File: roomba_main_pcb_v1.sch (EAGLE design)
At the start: 14 parts, among them J1 J25MM

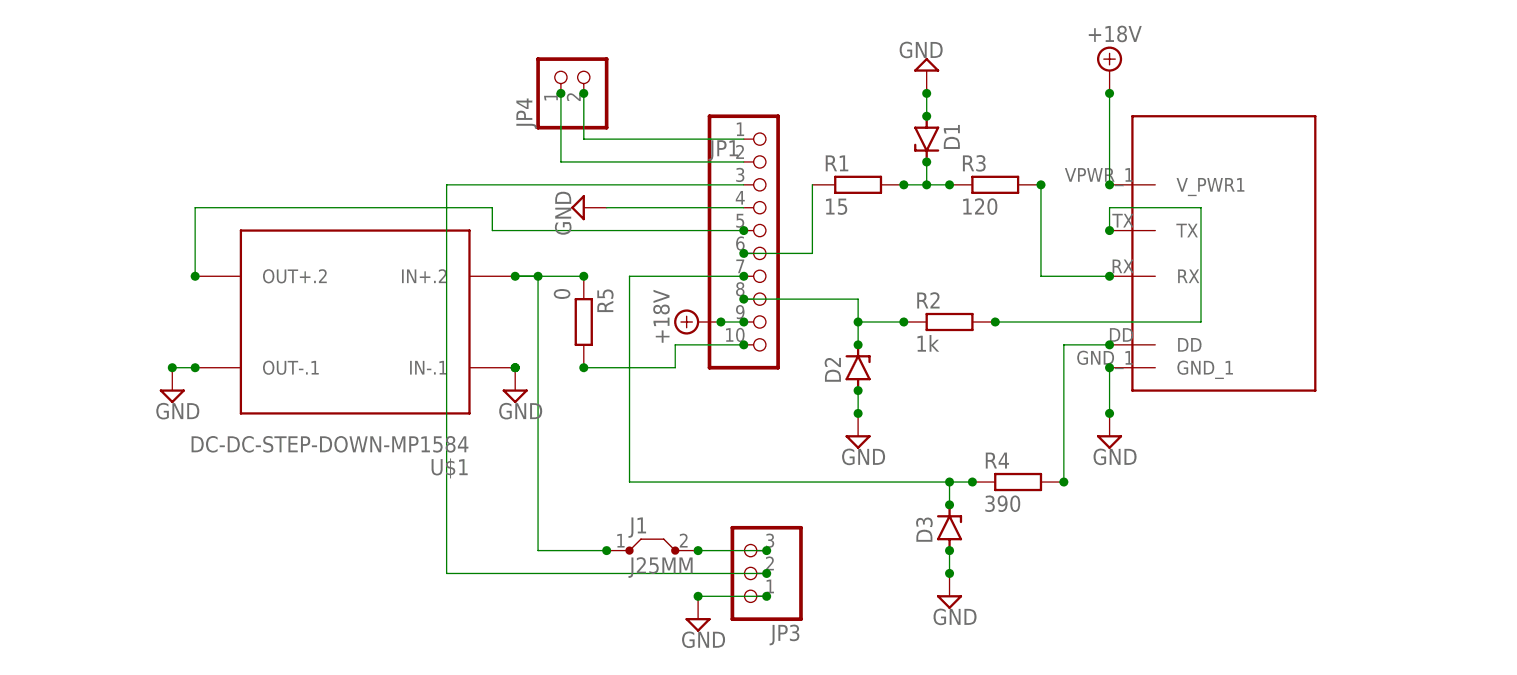
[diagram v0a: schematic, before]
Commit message: 1.1
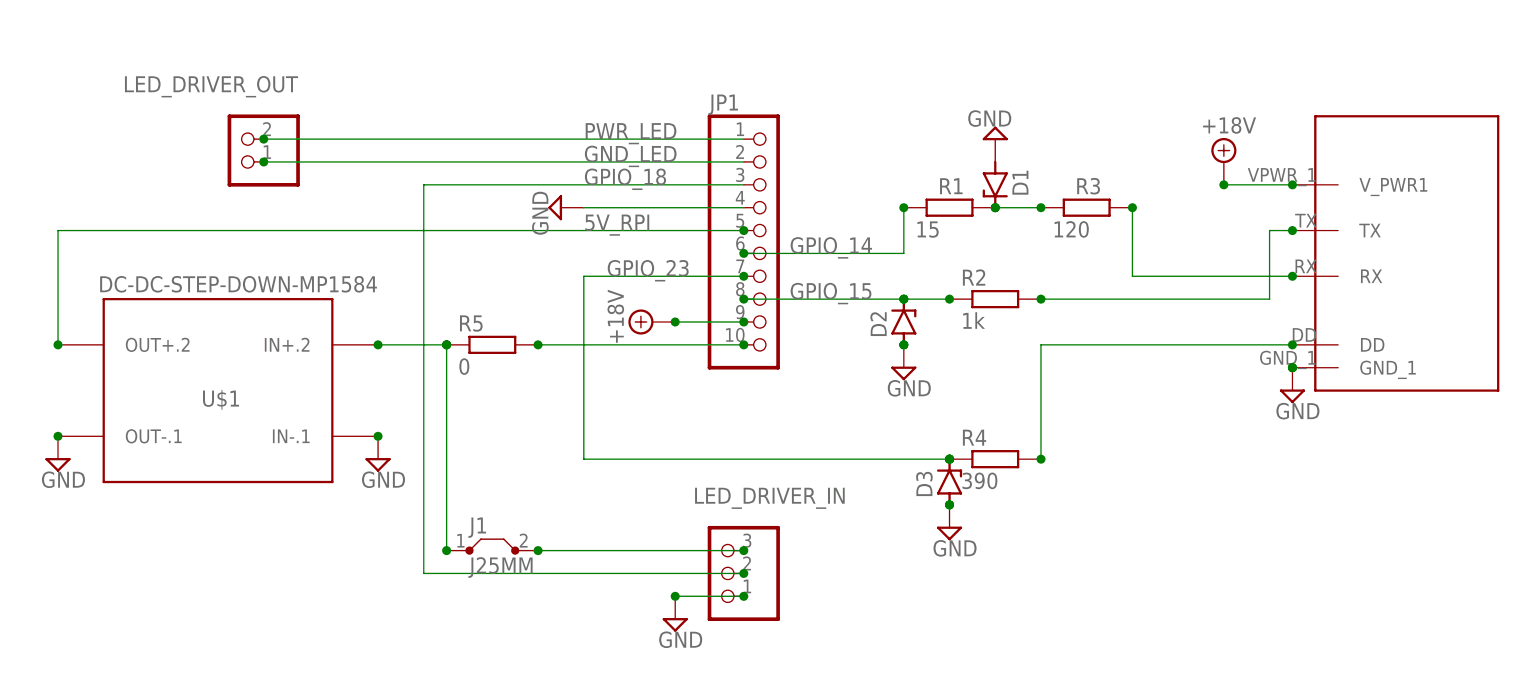
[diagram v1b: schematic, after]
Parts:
- removed JP3: (no value), pinhead:PINHD-1X3
- removed JP4: (no value), pinhead:PINHD-1X2
- removed U$3: 7_PIN, M_wifi:7_PIN
- added LED_DRIVER_IN: (no value), pinhead:PINHD-1X3
- added LED_DRIVER_OUT: (no value), pinhead:PINHD-1X2
- added ROOMBA_PORT: 7_PIN, M_wifi:7_PIN
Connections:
- net N$1 renamed GPIO_23
- net N$10 renamed 5V_RPI
- net N$14 renamed GPIO_14
- net N$3 renamed GPIO_15
- removed net N$12: JP1.3, JP3.2
- removed net N$13: JP1.1, JP4.2
- removed net N$15: JP1.2, JP4.1
- new net GND_LED: JP1.2, LED_DRIVER_OUT.1
- new net GPIO_18: JP1.3, LED_DRIVER_IN.2
- new net PWR_LED: JP1.1, LED_DRIVER_OUT.2
- net +18V: now also ROOMBA_PORT.V_PWR1; no longer U$3.V_PWR1
- net GND: now also LED_DRIVER_IN.1, ROOMBA_PORT.GND_1; no longer JP3.1, U$3.GND_1
- net N$5: now also ROOMBA_PORT.DD; no longer U$3.DD
- net N$6: now also LED_DRIVER_IN.3; no longer JP3.3
- net N$7: now also ROOMBA_PORT.RX; no longer U$3.RX
- net N$9: now also ROOMBA_PORT.TX; no longer U$3.TX
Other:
- moved on the sheet: D1, D2, D3, J1, R1, R2, R3, R4, R5, U$1
